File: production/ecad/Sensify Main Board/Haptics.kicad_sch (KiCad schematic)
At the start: 16 parts, among them J10 Conn_01x02_Socket, J4 Conn_01x02_Socket, J8 Conn_01x02_Socket, J9 Conn_01x02_Socket, U1 DRV2605LDGSR, U2 DRV2605LDGSR, U3 DRV2605LDGSR, U4 DRV2605LDGSR

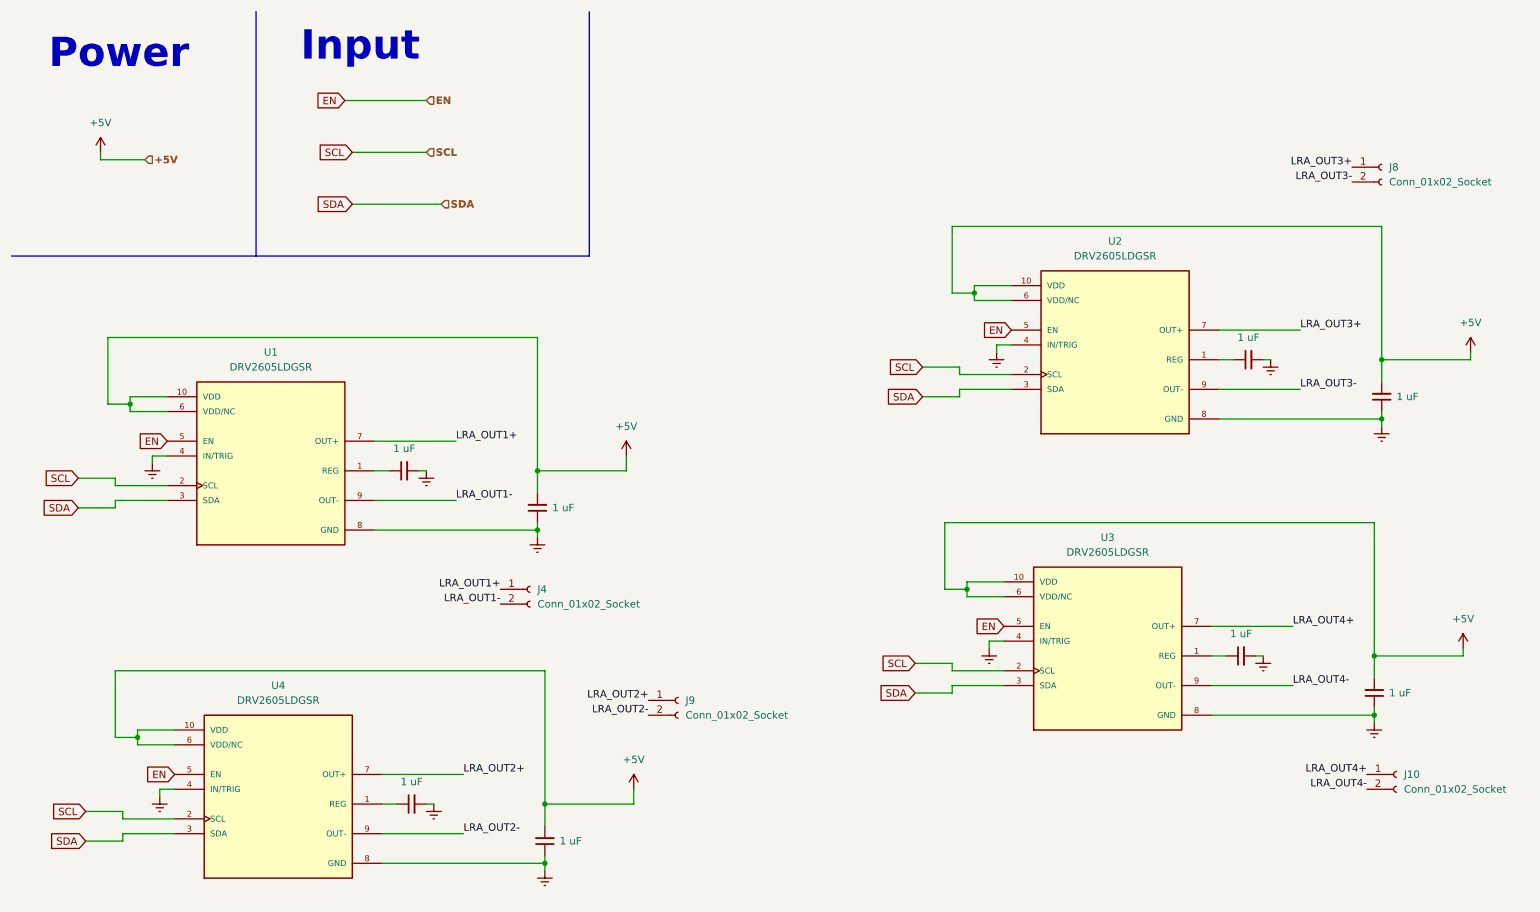
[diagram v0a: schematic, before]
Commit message: Finished IMU, Haptics, MCU, and Root Page
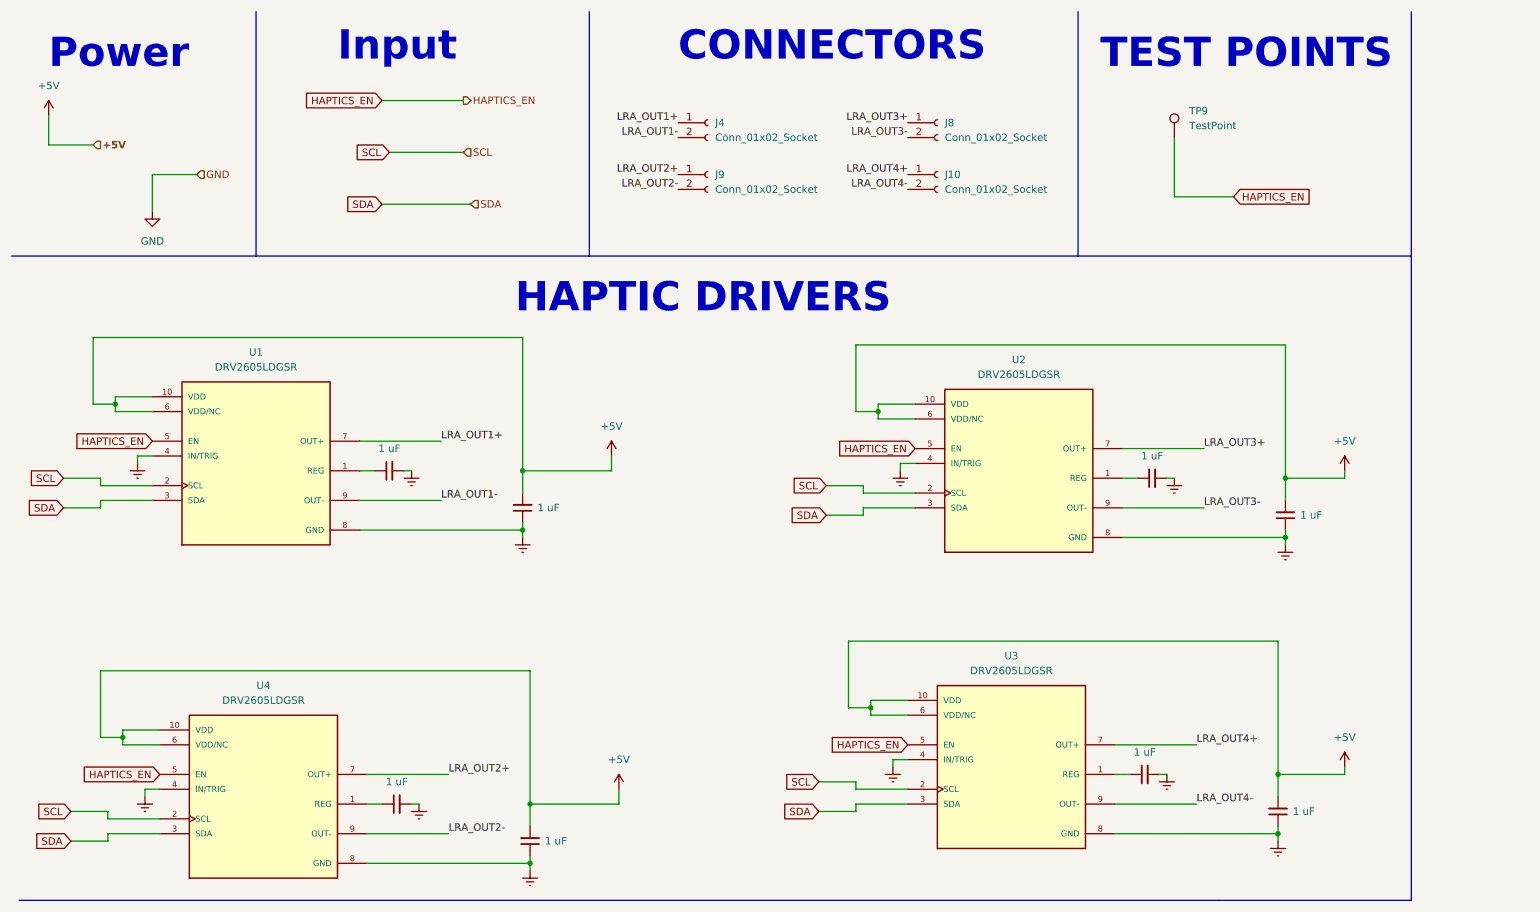
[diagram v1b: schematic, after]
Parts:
- added TP9: TestPoint, symbol Connector:TestPoint
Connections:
- net EN renamed HAPTICS_EN
- net HAPTICS_EN: now also TP9.1
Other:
- note added: "CONNECTORS"
- note added: "HAPTIC DRIVERS"
- note added: "TEST POINTS"
- moved on the sheet: J10, J4, J8, J9, U1, U2, U3, U4
